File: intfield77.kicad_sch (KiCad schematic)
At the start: 20 parts, among them J1 USB_C_Receptacle, SW1 RESET, SW2 BOOT, U1 STM32F072C8Tx, U2 SRV05-4, U3 XC6206PxxxMR

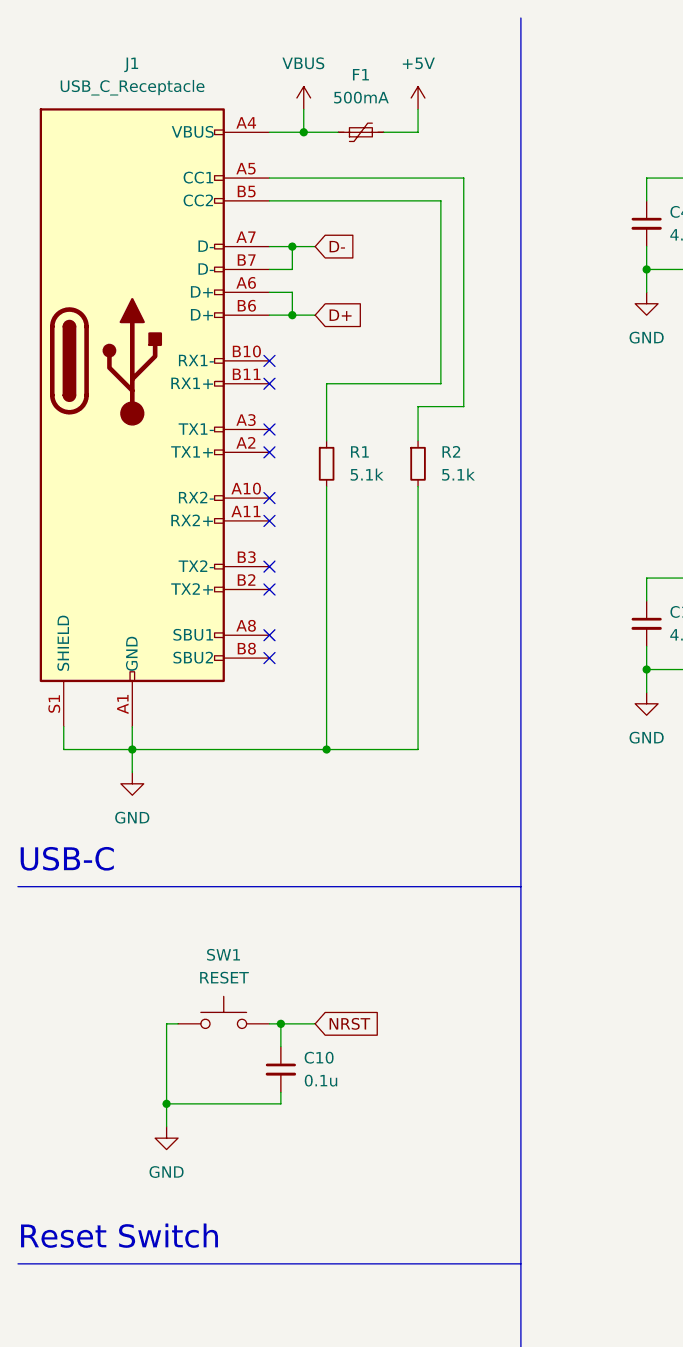
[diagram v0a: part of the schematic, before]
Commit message: Fixed it, I think.
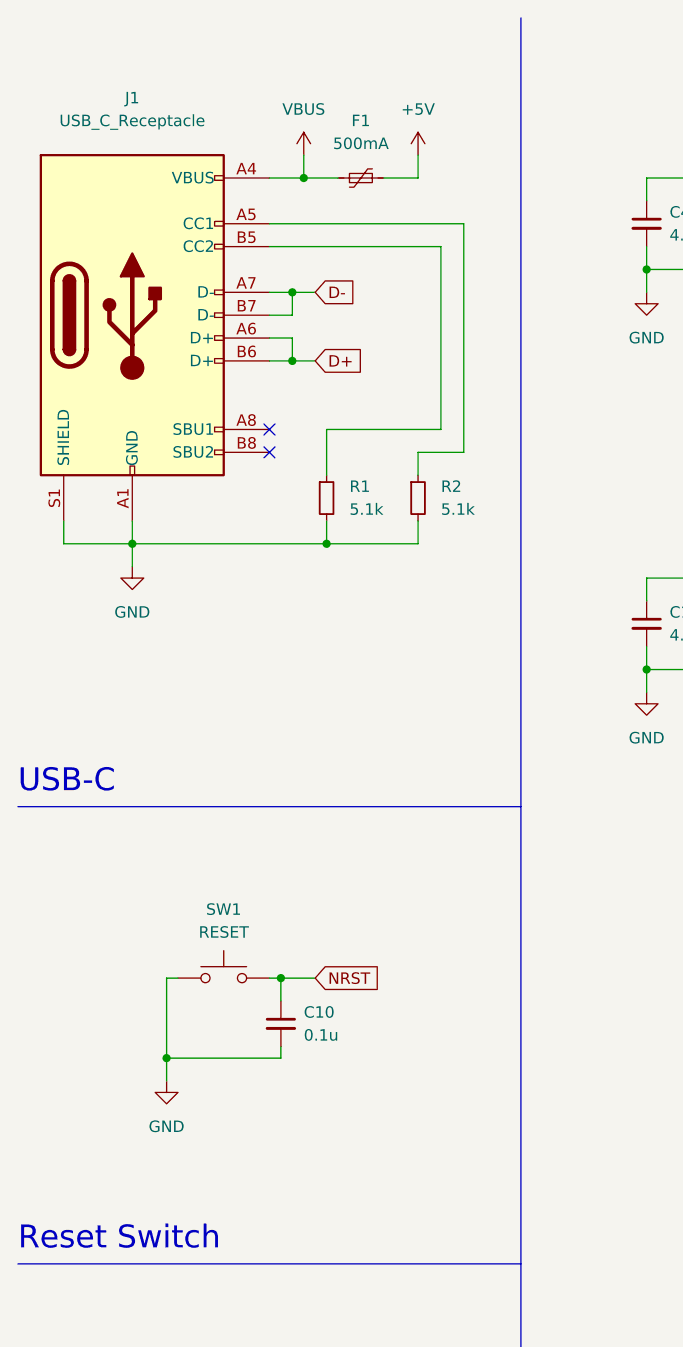
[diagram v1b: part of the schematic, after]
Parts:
- J1: symbol Connector:USB_C_Receptacle -> Connector:USB_C_Receptacle_USB2.0
- SW1: footprint Button_Switch_SMD:SW_Push_SPST_NO_Alps_SKRK -> Button_Switch_SMD:SW_SPST_SKQG_WithStem
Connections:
- no-connect marks 24 -> 16
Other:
- moved on the sheet: C10, F1, R1, R2, SW1
